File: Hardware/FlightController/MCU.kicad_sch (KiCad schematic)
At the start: 25 parts, among them J1 Conn_01x03, Q1 MMBT3904, SW1 SW_SPDT, U1 STM32F405RGT6, U2 USBLC6-2SC6, U3 W25Q128JVS, Y1 16MHz

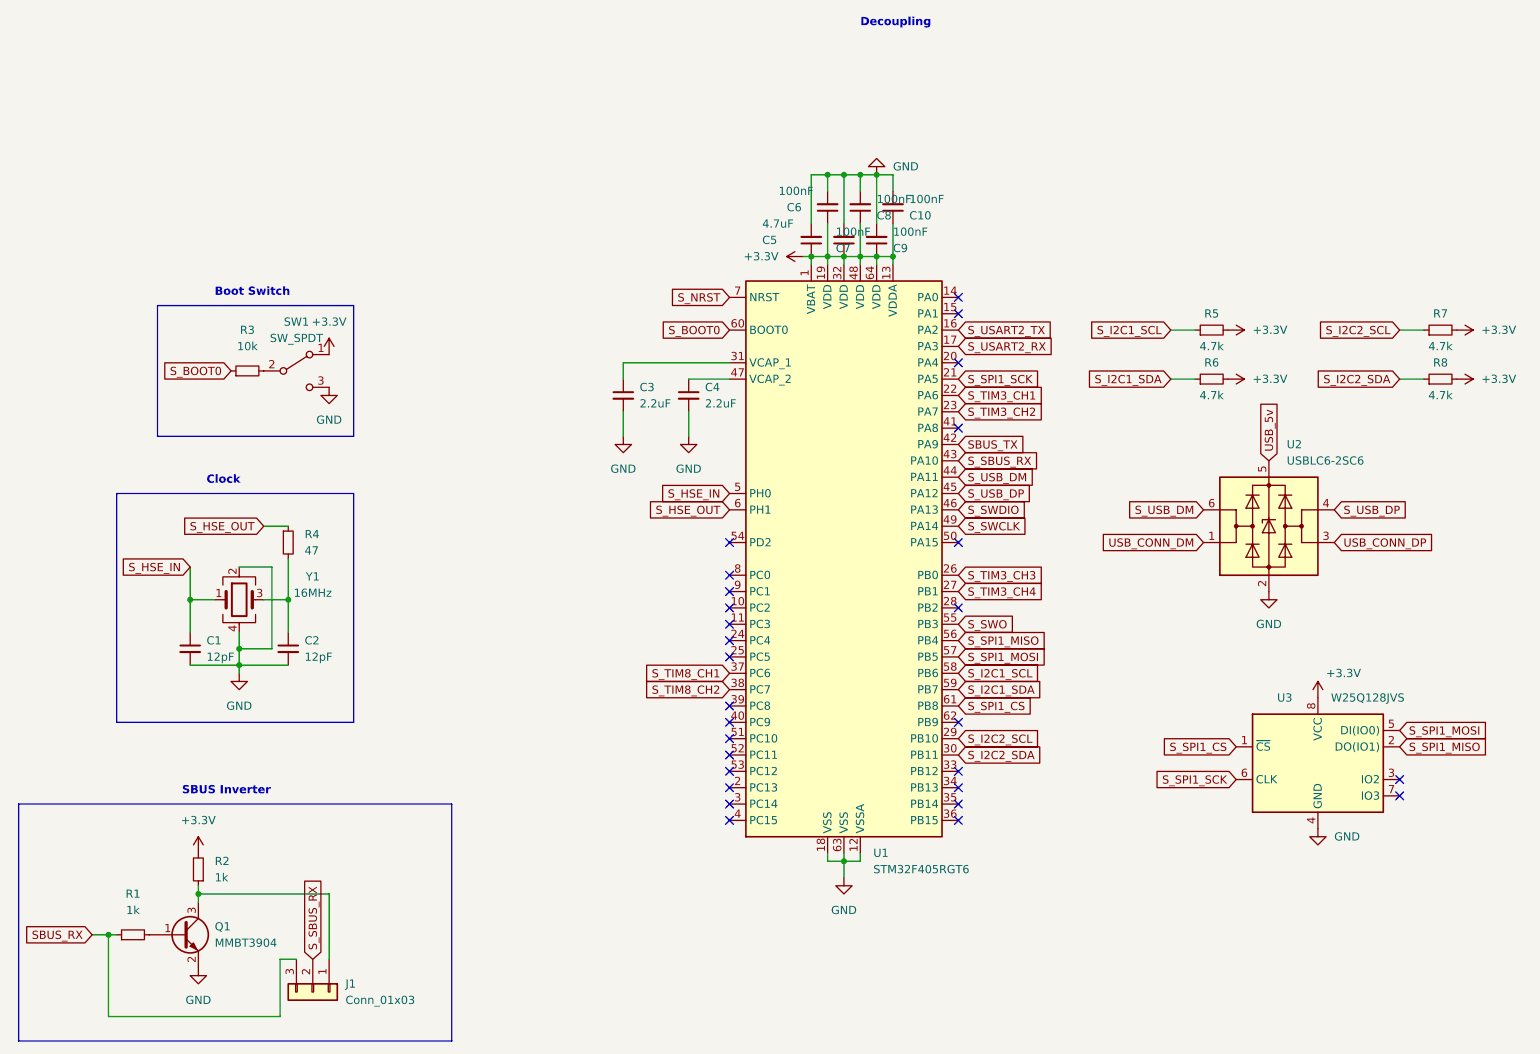
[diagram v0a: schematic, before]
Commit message: Finalize design and routing for v1.0 fab
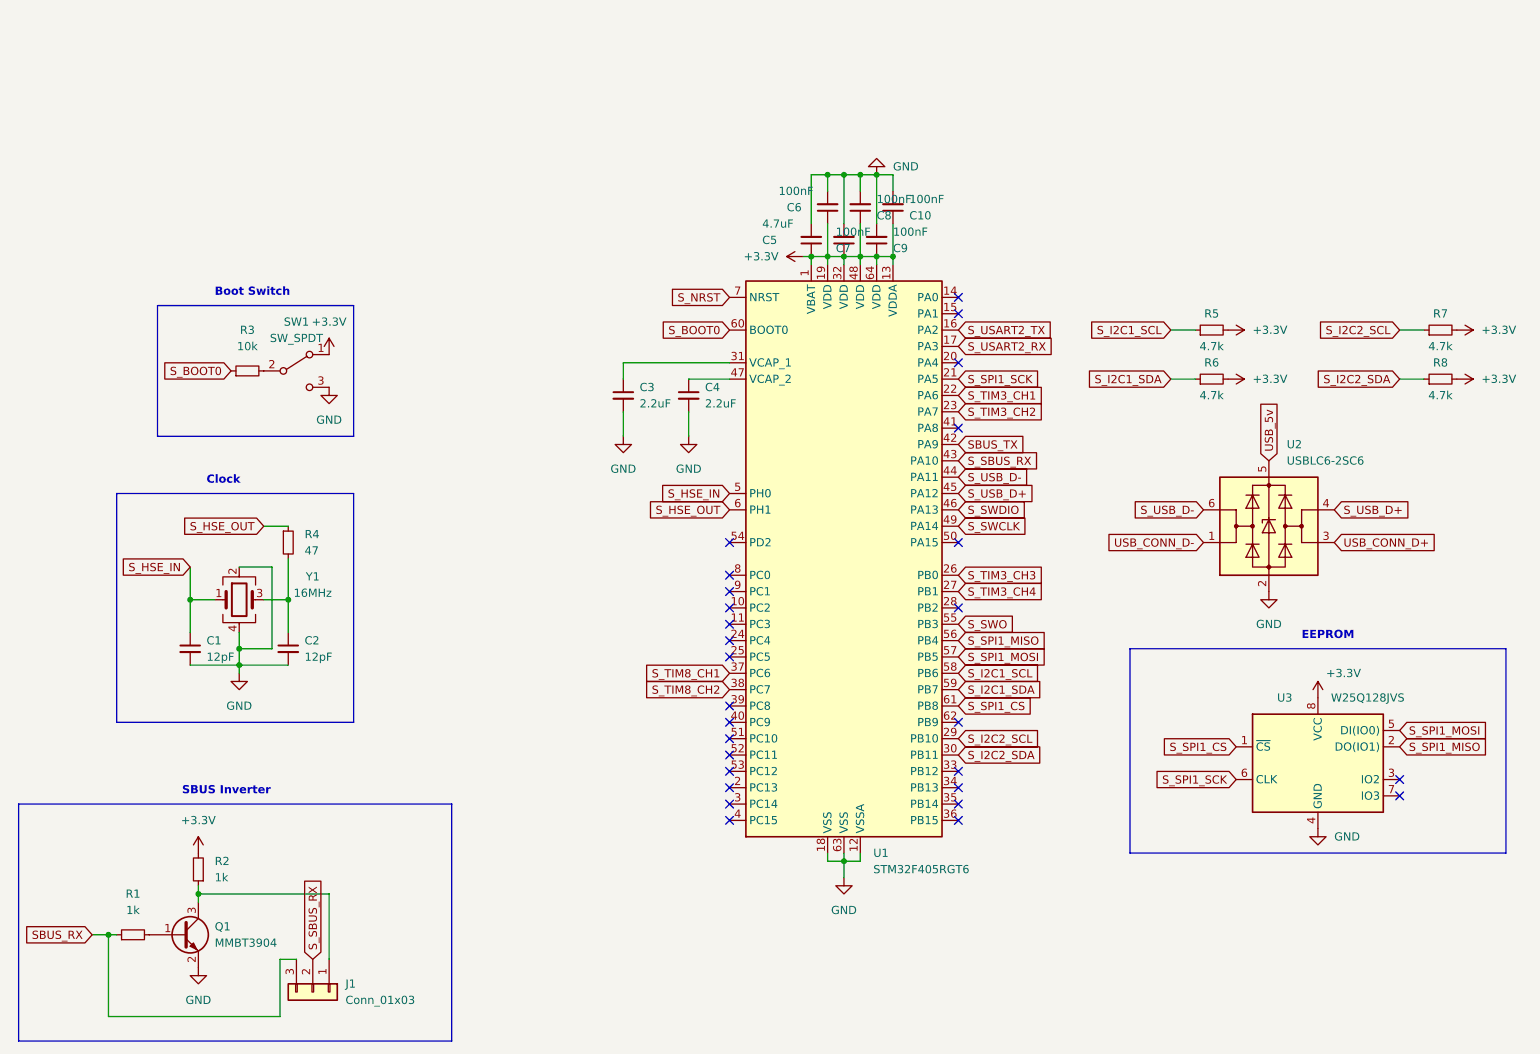
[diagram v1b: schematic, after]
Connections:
- net S_USB_DM renamed S_USB_D-
- net S_USB_DP renamed S_USB_D+
- net USB_CONN_DM renamed USB_CONN_D-
- net USB_CONN_DP renamed USB_CONN_D+
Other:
- note added: "EEPROM"
- note removed: "Decoupling"
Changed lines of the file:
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@@
+    (stroke (width 0) (type default) (color 0 0 0 0))
+  )
+  (polyline (pts (xy 256.54 121.92) (xy 256.54 153.67))
     (stroke (width 0) (type default) (color 0 0 0 0))
   )
@@
     (stroke (width 0) (type default) (color 0 0 0 0))
   )
+  (polyline (pts (xy 198.12 121.92) (xy 256.54 121.92))
+    (stroke (width 0) (type default) (color 0 0 0 0))
+  )
   (wire (pts (xy 153.67 153.67) (xy 153.67 154.94))
     (stroke (width 0) (type default) (color 0 0 0 0))
@@
     (stroke (width 0) (type default) (color 0 0 0 0))
   )
+  (polyline (pts (xy 198.12 153.67) (xy 198.12 121.92))
+    (stroke (width 0) (type default) (color 0 0 0 0))
+  )
   (wire (pts (xy 52.07 114.3) (xy 52.07 119.38))
     (stroke (width 0) (type default) (color 0 0 0 0))
@@
   )
   (wire (pts (xy 161.29 55.88) (xy 161.29 60.96))
+    (stroke (width 0) (type default) (color 0 0 0 0))
+  )
+  (polyline (pts (xy 256.54 153.67) (xy 198.12 153.67))
     (stroke (width 0) (type default) (color 0 0 0 0))
   )
@@
     (effects (font (size 1.27 1.27) bold) (justify left bottom))
   )
-  (text "Decoupling" (at 156.21 25.4 0)
+  (text "EEPROM" (at 224.79 120.65 0)
     (effects (font (size 1.27 1.27) bold) (justify left bottom))
   )
@@
     )
   )
-  (global_label "USB_CONN_DP" (shape input) (at 229.87 105.41 0) (fields_autoplaced)
-    (effects (font (size 1.27 1.27)) (justify left))
-    (property "Intersheet References" "${INTERSHEET_REFS}" (id 0) (at 245.8298 105.3306 0)
+  (global_label "USB_CONN_D+" (shape input) (at 229.87 105.41 0) (fields_autoplaced)
+    (effects (font (size 1.27 1.27)) (justify left))
+    (property "Intersheet References" "${INTERSHEET_REFS}" (id 0) (at 246.1321 105.3306 0)
       (effects (font (size 1.27 1.27)) (justify left) hide)
     )
@@
     )
   )
-  (global_label "S_USB_DP" (shape input) (at 229.87 100.33 0) (fields_autoplaced)
-    (effects (font (size 1.27 1.27)) (justify left))
-    (property "Intersheet References" "${INTERSHEET_REFS}" (id 0) (at 241.7779 100.2506 0)
-      (effects (font (size 1.27 1.27)) (justify left) hide)
-    )
-  )
-  (global_label "S_USB_DP" (shape input) (at 171.45 97.79 0) (fields_autoplaced)
-    (effects (font (size 1.27 1.27)) (justify left))
-    (property "Intersheet References" "${INTERSHEET_REFS}" (id 0) (at 183.3579 97.7106 0)
+  (global_label "S_USB_D+" (shape input) (at 229.87 100.33 0) (fields_autoplaced)
+    (effects (font (size 1.27 1.27)) (justify left))
+    (property "Intersheet References" "${INTERSHEET_REFS}" (id 0) (at 242.0802 100.2506 0)
+      (effects (font (size 1.27 1.27)) (justify left) hide)
+    )
+  )
+  (global_label "S_USB_D+" (shape input) (at 171.45 97.79 0) (fields_autoplaced)
+    (effects (font (size 1.27 1.27)) (justify left))
+    (property "Intersheet References" "${INTERSHEET_REFS}" (id 0) (at 183.6602 97.7106 0)
       (effects (font (size 1.27 1.27)) (justify left) hide)
     )
@@
     )
   )
-  (global_label "USB_CONN_DM" (shape input) (at 209.55 105.41 180) (fields_autoplaced)
-    (effects (font (size 1.27 1.27)) (justify right))
-    (property "Intersheet References" "${INTERSHEET_REFS}" (id 0) (at 193.4088 105.3306 0)
+  (global_label "USB_CONN_D-" (shape input) (at 209.55 105.41 180) (fields_autoplaced)
+    (effects (font (size 1.27 1.27)) (justify right))
+    (property "Intersheet References" "${INTERSHEET_REFS}" (id 0) (at 193.2879 105.3306 0)
       (effects (font (size 1.27 1.27)) (justify right) hide)
     )
@@
     )
   )
-  (global_label "S_USB_DM" (shape input) (at 209.55 100.33 180) (fields_autoplaced)
-    (effects (font (size 1.27 1.27)) (justify right))
-    (property "Intersheet References" "${INTERSHEET_REFS}" (id 0) (at 197.4607 100.4094 0)
+  (global_label "S_USB_D-" (shape input) (at 209.55 100.33 180) (fields_autoplaced)
+    (effects (font (size 1.27 1.27)) (justify right))
+    (property "Intersheet References" "${INTERSHEET_REFS}" (id 0) (at 197.3398 100.2506 0)
       (effects (font (size 1.27 1.27)) (justify right) hide)
     )
@@
     )
   )
-  (global_label "S_USB_DM" (shape input) (at 171.45 95.25 0) (fields_autoplaced)
-    (effects (font (size 1.27 1.27)) (justify left))
-    (property "Intersheet References" "${INTERSHEET_REFS}" (id 0) (at 183.5393 95.1706 0)
-      (effects (font (size 1.27 1.27)) (justify left) hide)
-    )
+  (global_label "S_USB_D-" (shape input) (at 171.45 95.25 0) (fields_autoplaced)
+    (effects (font (size 1.27 1.27)) (justify left))
+    (property "Intersheet References" "${INTERSHEET_REFS}" (id 0) (at 183.6602 95.1706 0)
+      (effects (font (size 1.27 1.27)) (justify left) hide)
+    )
